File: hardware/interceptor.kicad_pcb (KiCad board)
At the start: 2 copper layers, 80 x 59.7 mm, 28 parts, among them IC1 ATMEGA1284P-P, P1 TAPEPORT, P2 CIA1, P3 KEYBOARD, P4 USER, P6 USB, SW1 RESET, SW2 BOOTLOADER, U1 7400, U2 ICL7660, U3 4520, U4 4051, U5 4051, U6 CD74HC22106, X1 16Mhz

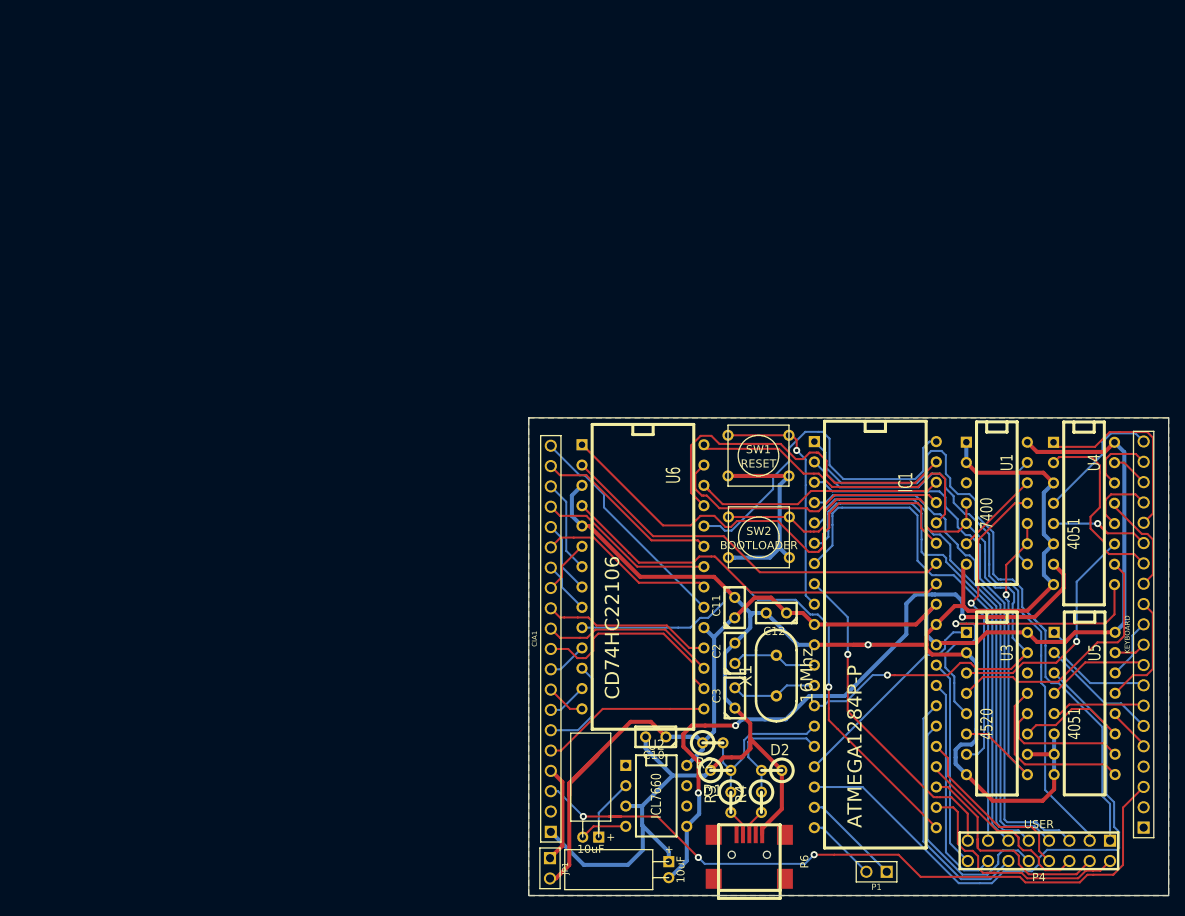
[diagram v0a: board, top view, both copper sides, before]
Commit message: Hardware: Revision 1
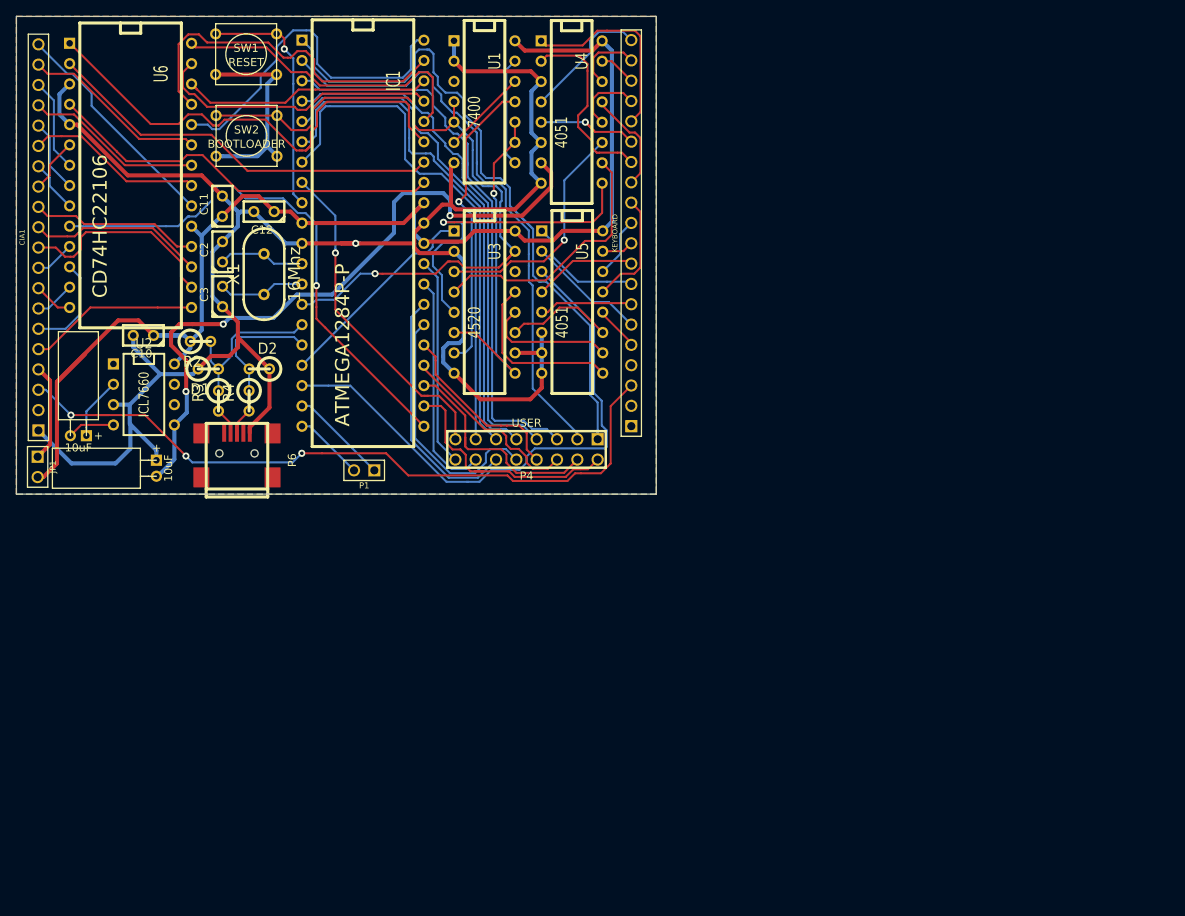
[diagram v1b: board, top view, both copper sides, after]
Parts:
- moved C3 81.4 mm to (130.4, 103.9)
- moved JP1 81.4 mm to (107.3, 125.2)
- moved U1 81.4 mm to (163.1, 79.5)
- moved C11 81.4 mm to (130.4, 92.6)
- moved C2 81.4 mm to (130.4, 98.3)
- moved IC1 81.4 mm to (147.9, 96.0)
- moved P1 81.4 mm to (148.1, 125.6)
- moved P6 81.4 mm to (132.2, 124.3)
- moved R3 81.4 mm to (129.9, 116.9)
- moved SW2 81.4 mm to (133.4, 83.8)
- moved U2 81.4 mm to (120.6, 116.1)
- moved U5 81.4 mm to (174.1, 104.6)
- moved C10 81.4 mm to (120.5, 108.8)
- moved C12 81.4 mm to (135.6, 93.3)
- moved C4 81.4 mm to (112.4, 121.3)
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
